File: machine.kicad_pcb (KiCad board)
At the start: 2 copper layers, 69.8 x 69.8 mm, 34 parts, among them J1 TMC2209 Y, J10 SD Card, J11 Stop, J12 Serial, J13 STM32DevV1-VCC, J14 STM32DevV1-3.3, J2 TMC2209 B, J3 X Motor, J4 Y Motor, J5 24V, J6 Buttons, J7 X limit, J8 Y limit, J9 Display, U2 K7805W-500R3

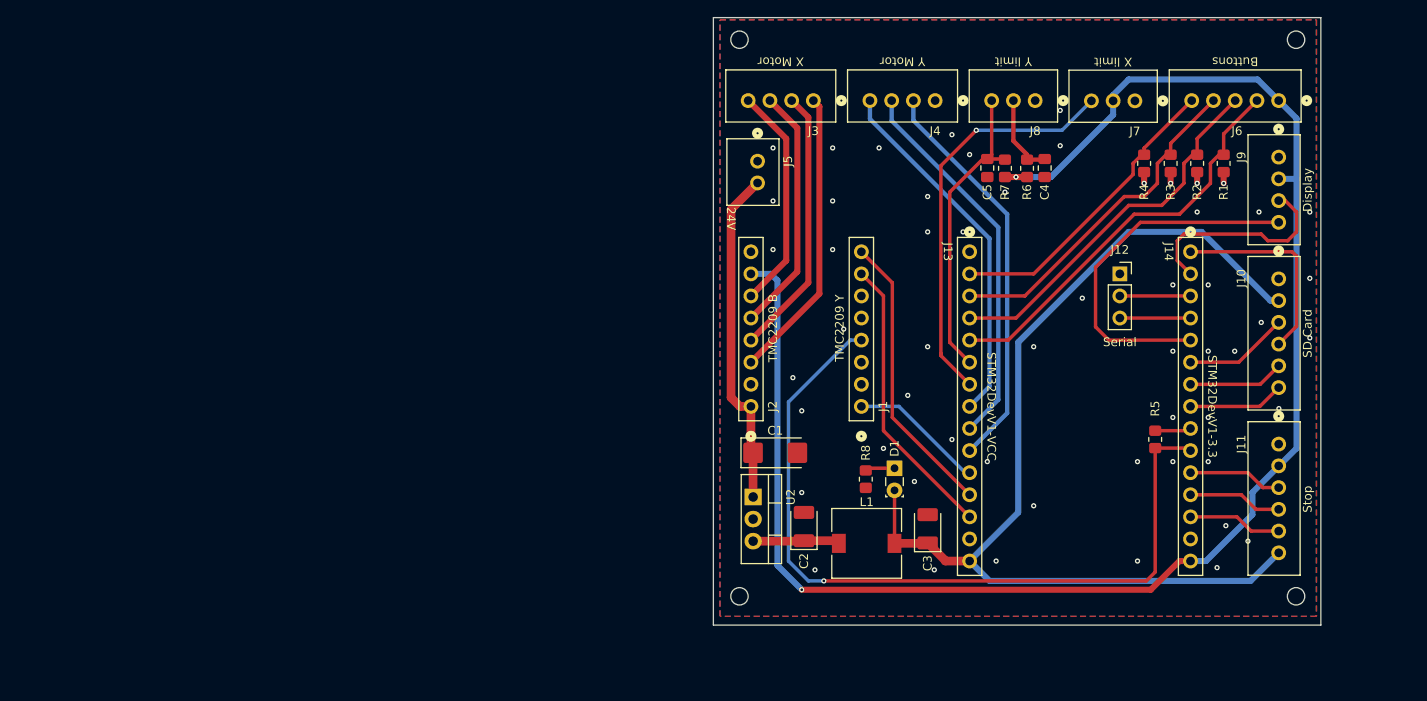
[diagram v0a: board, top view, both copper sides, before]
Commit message: Finalization v2.0
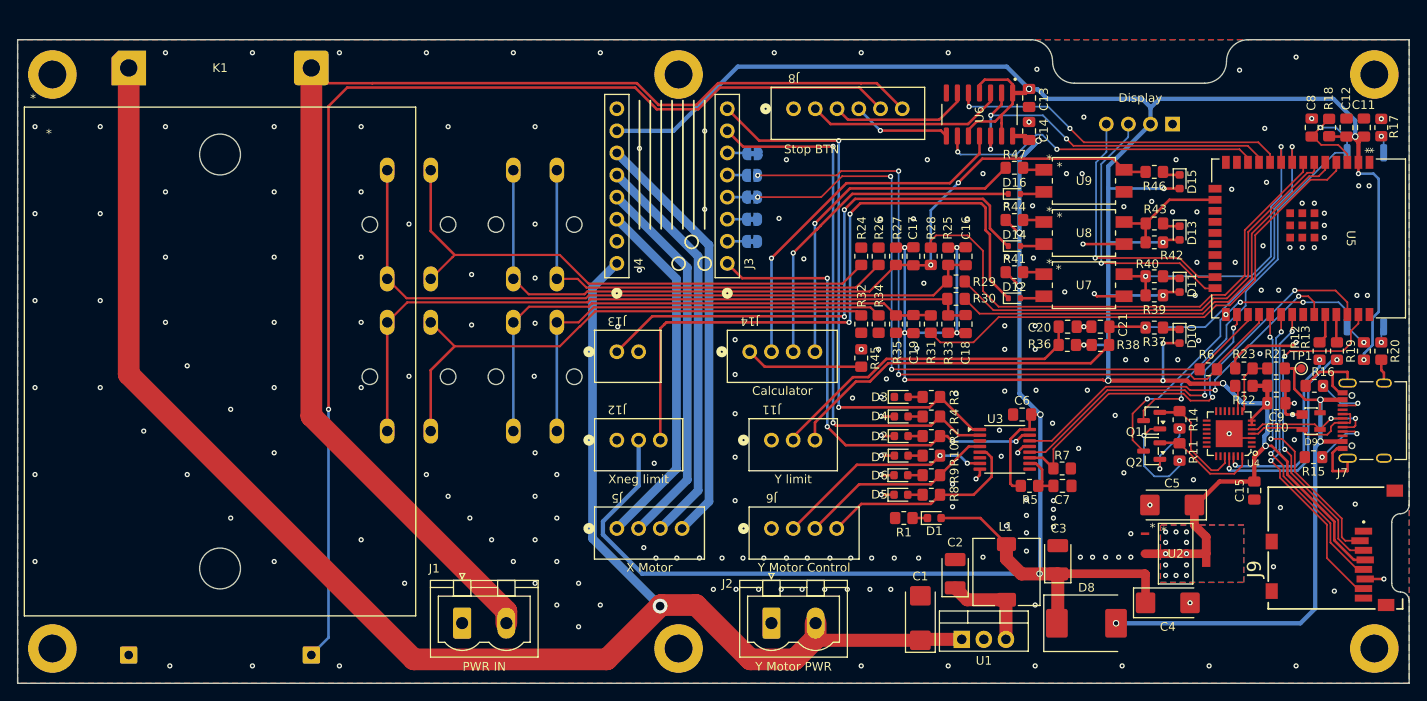
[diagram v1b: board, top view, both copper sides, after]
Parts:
- removed REF** (x4): MountingHole_2mm, MountingHole:MountingHole_2mm
- added C10: 10μF, Capacitor_SMD:C_0805_2012Metric_Pad1.18x1.45mm_HandSolder, F.Cu at (201.7, 86.3)
- added C11: 100nF, Capacitor_SMD:C_0805_2012Metric_Pad1.18x1.45mm_HandSolder, F.Cu at (211.8, 54.6)
- added C12: 22μF, Capacitor_SMD:C_0805_2012Metric_Pad1.18x1.45mm_HandSolder, F.Cu at (209.8, 54.6)
- added C13: 100nF, Capacitor_SMD:C_0805_2012Metric_Pad1.18x1.45mm_HandSolder, F.Cu at (173.3, 51.2)
- added C14: 100nF, Capacitor_SMD:C_0805_2012Metric_Pad1.18x1.45mm_HandSolder, F.Cu at (173.3, 55.0)
- added C15: 100nF, Capacitor_SMD:C_0805_2012Metric_Pad1.18x1.45mm_HandSolder, F.Cu at (199.2, 96.3)
- added C16: 100nF, Capacitor_SMD:C_0805_2012Metric_Pad1.18x1.45mm_HandSolder, F.Cu at (166.0, 69.4)
- added C17: 100nF, Capacitor_SMD:C_0805_2012Metric_Pad1.18x1.45mm_HandSolder, F.Cu at (160.0, 69.4)
- added C18: 100nF, Capacitor_SMD:C_0805_2012Metric_Pad1.18x1.45mm_HandSolder, F.Cu at (166.0, 77.2)
- added C19: 100nF, Capacitor_SMD:C_0805_2012Metric_Pad1.18x1.45mm_HandSolder, F.Cu at (160.0, 77.2)
- added C20: 4.7nF, Capacitor_SMD:C_0805_2012Metric_Pad1.18x1.45mm_HandSolder, F.Cu at (177.7, 77.5)
- added C21: 4.7nF, Capacitor_SMD:C_0805_2012Metric_Pad1.18x1.45mm_HandSolder, F.Cu at (181.5, 77.5)
- added C6: 100nF, Capacitor_SMD:C_0805_2012Metric_Pad1.18x1.45mm_HandSolder, F.Cu at (172.5, 87.6)
- added C7: 100nF, Capacitor_SMD:C_0805_2012Metric_Pad1.18x1.45mm_HandSolder, F.Cu at (177.1, 95.8)
- added C8: 100nF, Capacitor_SMD:C_0805_2012Metric_Pad1.18x1.45mm_HandSolder, F.Cu at (205.8, 54.6)
- added C9: 100nF, Capacitor_SMD:C_0805_2012Metric_Pad1.18x1.45mm_HandSolder, F.Cu at (201.7, 84.3)
- added D10: LED, LED_SMD:LED_0603_1608Metric, F.Cu at (190.6, 78.6)
- added D11: LED, LED_SMD:LED_0603_1608Metric, F.Cu at (190.6, 72.7)
- added D12: RB521S30, Diode_SMD:D_SOD-523, F.Cu at (171.6, 74.2)
- added D13: LED, LED_SMD:LED_0603_1608Metric, F.Cu at (190.6, 66.7)
- added D14: RB521S30, Diode_SMD:D_SOD-523, F.Cu at (171.6, 68.2)
- added D15: LED, LED_SMD:LED_0603_1608Metric, F.Cu at (190.6, 60.8)
- added D16: RB521S30, Diode_SMD:D_SOD-523, F.Cu at (171.6, 62.2)
- added D2: LED, LED_SMD:LED_0603_1608Metric, F.Cu at (158.6, 90.1)
- added D3: LED, LED_SMD:LED_0603_1608Metric, F.Cu at (158.6, 85.6)
- added D4: LED, LED_SMD:LED_0603_1608Metric, F.Cu at (158.6, 87.8)
- added D5: LED, LED_SMD:LED_0603_1608Metric, F.Cu at (158.6, 96.8)
- added D6: LED, LED_SMD:LED_0603_1608Metric, F.Cu at (158.6, 94.6)
- added D7: LED, LED_SMD:LED_0603_1608Metric, F.Cu at (158.6, 92.3)
- added D8: B340A-13-F, Diode_SMD:D_SMC, F.Cu at (179.9, 111.6)
- added D9: SP0503BAHTG, SP0503BAHTG:SOT143, F.Cu at (205.7, 88.4)
- added H1: ~, MountingHole:MountingHole_3.2mm_M3_DIN965_Pad, F.Cu at (61.0, 48.5)
- added H2: ~, MountingHole:MountingHole_3.2mm_M3_DIN965_Pad, F.Cu at (133.0, 48.5)
- added H3: ~, MountingHole:MountingHole_3.2mm_M3_DIN965_Pad, F.Cu at (213.0, 48.5)
- added H4: ~, MountingHole:MountingHole_3.2mm_M3_DIN965_Pad, F.Cu at (213.0, 114.5)
- added H5: ~, MountingHole:MountingHole_3.2mm_M3_DIN965_Pad, F.Cu at (133.0, 114.5)
- added H6: ~, MountingHole:MountingHole_3.2mm_M3_DIN965_Pad, F.Cu at (61.0, 114.5)
- added JP1: PDN, Jumper:SolderJumper-2_P1.3mm_Bridged_RoundedPad1.0x1.5mm, B.Cu at (141.4, 62.6)
- added JP2: PDN, Jumper:SolderJumper-2_P1.3mm_Open_RoundedPad1.0x1.5mm, B.Cu at (141.4, 60.1)
- added JP3: CK, Jumper:SolderJumper-2_P1.3mm_Bridged_RoundedPad1.0x1.5mm, B.Cu at (141.5, 57.6)
- added JP4: MS1, Jumper:SolderJumper-2_P1.3mm_Bridged_RoundedPad1.0x1.5mm, B.Cu at (141.4, 67.7)
- added JP5: MS2, Jumper:SolderJumper-2_P1.3mm_Bridged_RoundedPad1.0x1.5mm, B.Cu at (141.4, 65.2)
- added K1: ZGT-40DD, SSR-DCDC:SSR_DCDC, F.Cu at (57.8, 52.2)
- added Q1: SS8050, Package_TO_SOT_SMD:SOT-23, F.Cu at (187.4, 88.3)
- added Q2: SS8050, Package_TO_SOT_SMD:SOT-23, F.Cu at (187.4, 91.8)
- added R10: 10k, Resistor_SMD:R_0805_2012Metric_Pad1.20x1.40mm_HandSolder, F.Cu at (162.1, 92.3)
- added R11: 10k, Resistor_SMD:R_0805_2012Metric_Pad1.20x1.40mm_HandSolder, F.Cu at (190.6, 91.9)
- added R12: 0, Resistor_SMD:R_0805_2012Metric_Pad1.20x1.40mm_HandSolder, F.Cu at (206.7, 80.3)
- added R13: 0, Resistor_SMD:R_0805_2012Metric_Pad1.20x1.40mm_HandSolder, F.Cu at (208.7, 80.3)
- added R14: 10k, Resistor_SMD:R_0805_2012Metric_Pad1.20x1.40mm_HandSolder, F.Cu at (190.6, 88.2)
- added R15: 5.1k, Resistor_SMD:R_0805_2012Metric_Pad1.20x1.40mm_HandSolder, F.Cu at (206.0, 92.5)
- added R16: 5.1k, Resistor_SMD:R_0805_2012Metric_Pad1.20x1.40mm_HandSolder, F.Cu at (206.1, 84.3)
- added R17: 1k, Resistor_SMD:R_0805_2012Metric_Pad1.20x1.40mm_HandSolder, F.Cu at (213.8, 54.6)
- added R18: 10k, Resistor_SMD:R_0805_2012Metric_Pad1.20x1.40mm_HandSolder, F.Cu at (207.8, 54.6)
- added R19: 10k, Resistor_SMD:R_0805_2012Metric_Pad1.20x1.40mm_HandSolder, F.Cu at (211.8, 80.3)
- added R20: 1k, Resistor_SMD:R_0805_2012Metric_Pad1.20x1.40mm_HandSolder, F.Cu at (213.8, 80.3)
- added R21: 22.1k, Resistor_SMD:R_0805_2012Metric_Pad1.20x1.40mm_HandSolder, F.Cu at (201.7, 82.3)
- added R22: 2k, Resistor_SMD:R_0805_2012Metric_Pad1.20x1.40mm_HandSolder, F.Cu at (198.0, 84.3)
- added R23: 47.5k, Resistor_SMD:R_0805_2012Metric_Pad1.20x1.40mm_HandSolder, F.Cu at (198.0, 82.3)
- added R24: 10, Resistor_SMD:R_0805_2012Metric_Pad1.20x1.40mm_HandSolder, F.Cu at (154.0, 69.4)
- added R25: 1k, Resistor_SMD:R_0805_2012Metric_Pad1.20x1.40mm_HandSolder, F.Cu at (164.0, 69.4)
- added R26: 10, Resistor_SMD:R_0805_2012Metric_Pad1.20x1.40mm_HandSolder, F.Cu at (156.0, 69.4)
- added R27: 1k, Resistor_SMD:R_0805_2012Metric_Pad1.20x1.40mm_HandSolder, F.Cu at (158.0, 69.4)
- added R28: 33, Resistor_SMD:R_0805_2012Metric_Pad1.20x1.40mm_HandSolder, F.Cu at (162.0, 69.4)
- added R29: 33, Resistor_SMD:R_0805_2012Metric_Pad1.20x1.40mm_HandSolder, F.Cu at (164.9, 72.3)
- added R30: 33, Resistor_SMD:R_0805_2012Metric_Pad1.20x1.40mm_HandSolder, F.Cu at (164.9, 74.3)
- added R31: 33, Resistor_SMD:R_0805_2012Metric_Pad1.20x1.40mm_HandSolder, F.Cu at (162.0, 77.2)
- added R32: 10, Resistor_SMD:R_0805_2012Metric_Pad1.20x1.40mm_HandSolder, F.Cu at (154.0, 77.2)
- added R33: 1k, Resistor_SMD:R_0805_2012Metric_Pad1.20x1.40mm_HandSolder, F.Cu at (164.0, 77.2)
- added R34: 10, Resistor_SMD:R_0805_2012Metric_Pad1.20x1.40mm_HandSolder, F.Cu at (156.0, 77.2)
- added R35: 1k, Resistor_SMD:R_0805_2012Metric_Pad1.20x1.40mm_HandSolder, F.Cu at (158.0, 77.2)
- added R36: 200, Resistor_SMD:R_0805_2012Metric_Pad1.20x1.40mm_HandSolder, F.Cu at (177.7, 79.6)
- added R37: 6k8, Resistor_SMD:R_0805_2012Metric_Pad1.20x1.40mm_HandSolder, F.Cu at (187.7, 77.6)
- added R38: 1k2, Resistor_SMD:R_0805_2012Metric_Pad1.20x1.40mm_HandSolder, F.Cu at (181.5, 79.6)
- added R39: 10k, Resistor_SMD:R_0805_2012Metric_Pad1.20x1.40mm_HandSolder, F.Cu at (187.7, 73.9)
- added R40: 6k8, Resistor_SMD:R_0805_2012Metric_Pad1.20x1.40mm_HandSolder, F.Cu at (187.7, 71.7)
- added R41: 680, Resistor_SMD:R_0805_2012Metric_Pad1.20x1.40mm_HandSolder, F.Cu at (171.6, 71.2)
- added R42: 10k, Resistor_SMD:R_0805_2012Metric_Pad1.20x1.40mm_HandSolder, F.Cu at (187.7, 67.8)
- added R43: 6k8, Resistor_SMD:R_0805_2012Metric_Pad1.20x1.40mm_HandSolder, F.Cu at (187.7, 65.6)
- added R44: 680, Resistor_SMD:R_0805_2012Metric_Pad1.20x1.40mm_HandSolder, F.Cu at (171.6, 65.2)
- added R45: 680, Resistor_SMD:R_0805_2012Metric_Pad1.20x1.40mm_HandSolder, F.Cu at (154.0, 81.1)
- added R46: 6k8, Resistor_SMD:R_0805_2012Metric_Pad1.20x1.40mm_HandSolder, F.Cu at (187.7, 59.7)
- added R47: 0, Resistor_SMD:R_0805_2012Metric_Pad1.20x1.40mm_HandSolder, F.Cu at (171.6, 59.2)
- added R9: 10k, Resistor_SMD:R_0805_2012Metric_Pad1.20x1.40mm_HandSolder, F.Cu at (162.1, 94.6)
- added SW1: Reset, Button_Switch_SMD:SW_Push_SPST_NO_Alps_SKRK, B.Cu at (212.0, 57.5)
- added SW2: Boot, Button_Switch_SMD:SW_Push_SPST_NO_Alps_SKRK, B.Cu at (212.0, 77.5)
- added SW3: Run, Button_Switch_THT:SW_SPST_Omron_B3F-40xx, B.Cu at (99.5, 59.5)
- added SW4: Hold, Button_Switch_THT:SW_SPST_Omron_B3F-40xx, B.Cu at (114.0, 59.5)
- added SW5: M2, Button_Switch_THT:SW_SPST_Omron_B3F-40xx, B.Cu at (99.5, 77.0)
- added SW6: M1, Button_Switch_THT:SW_SPST_Omron_B3F-40xx, B.Cu at (114.0, 77.0)
- added TP1: ~, TestPoint:TestPoint_Pad_D1.0mm, F.Cu at (204.6, 82.3)
- added U1: K7805W-500R3, Package_TO_SOT_THT:TO-220-3_Vertical, F.Cu at (165.6, 113.5)
- added U3: 74AHCT595, Package_SO:TSSOP-16_4.4x5mm_P0.65mm, F.Cu at (170.5, 91.6)
- added U4: CP2102-GMR, CP2102_GMR:QFN28G_0.5-5X5MM, F.Cu at (196.3, 89.8)
- added U5: ESP32-WROOM-32E 4MB, ESP32-WROOM-32E-N4:ESP32-WROOM-32E_EXP, F.Cu at (207.2, 67.4)
- added U6: SN74LV125ADR, SN74LV125ADR:SOIC127P600X175-14N, F.Cu at (167.6, 53.1)
- added U7: TLP521-1, TLP521-1XSM:TLP521SM_ISO, F.Cu at (179.6, 72.7)
- added U8: TLP521-1, TLP521-1XSM:TLP521SM_ISO, F.Cu at (179.6, 66.7)
- added U9: TLP521-1, TLP521-1XSM:TLP521SM_ISO, F.Cu at (179.6, 60.7)
- C1: footprint Capacitor_Tantalum_SMD:CP_EIA-6032-28_Kemet-C_Pad2.25x2.35mm_HandSolder -> Capacitor_Tantalum_SMD:CP_EIA-6032-28_Kemet-C_HandSolder
- C2, C3: footprint Capacitor_Tantalum_SMD:CP_EIA-3528-21_Kemet-B_Pad1.50x2.35mm_HandSolder -> Capacitor_Tantalum_SMD:CP_EIA-3528-21_Kemet-B_HandSolder
- C4, C5: value 4.7nF -> 10μF; footprint Capacitor_SMD:C_0805_2012Metric_Pad1.18x1.45mm_HandSolder -> Capacitor_Tantalum_SMD:CP_EIA-6032-28_Kemet-C_HandSolder
- D1: footprint LED_THT:LED_Rectangular_W3.9mm_H1.9mm -> LED_SMD:LED_0603_1608Metric
- J1: value TMC2209 Y -> PWR IN; footprint HDR-08POS:CONN8_LFBN-RC_SUL -> Connector_Phoenix_MSTB:PhoenixContact_MSTBVA_2,5_2-G-5,08_1x02_P5.08mm_Vertical
- J10: value SD Card -> Display; footprint JST-XH-6A:CONN_B6B-XH-A_JST -> Connector_PinSocket_2.54mm:PinSocket_1x04_P2.54mm_Vertical; moved to B.Cu
- J11: value Stop -> Y limit; footprint JST-XH-6A:CONN_B6B-XH-A_JST -> JST-XH-3A:CONN_B3B-XH-A_JST
- J12: value Serial -> Xneg limit; footprint Connector_PinSocket_2.54mm:PinSocket_1x03_P2.54mm_Vertical -> JST-XH-3A:CONN_B3B-XH-A_JST
- J13: value STM32DevV1-VCC -> Xpos limit; footprint HDR-15POS:CONN15_PPPC151LFBN-RC_SUL -> JST-XH-2A:CONN_B2B-XH-A_JST
- J14: value STM32DevV1-3.3 -> Calculator; footprint HDR-15POS:CONN15_PPPC151LFBN-RC_SUL -> JST-XH-4A:CONN_B4B-XH-A_JST
- J2: value TMC2209 B -> Y Motor PWR; footprint HDR-08POS:CONN8_LFBN-RC_SUL -> Connector_Phoenix_MSTB:PhoenixContact_MSTBVA_2,5_2-G-5,08_1x02_P5.08mm_Vertical
- J3: value X Motor -> TMC2209 Y; footprint JST-XH-4A:CONN_B4B-XH-A_JST -> HDR-08POS:CONN8_LFBN-RC_SUL
- J4: value Y Motor -> TMC2209 B; footprint JST-XH-4A:CONN_B4B-XH-A_JST -> HDR-08POS:CONN8_LFBN-RC_SUL
- J5: value 24V -> X Motor; footprint JST-XH-2A:CONN_B2B-XH-A_JST -> JST-XH-4A:CONN_B4B-XH-A_JST
- J6: value Buttons -> Y Motor Control; footprint JST-XH-5A:CONN_B5B-XH-A_JST -> JST-XH-4A:CONN_B4B-XH-A_JST
- J7: value X limit -> TYPE-C 15PIN; footprint JST-XH-3A:CONN_B3B-XH-A_JST -> 10155435_00011LF:AMPHENOL_10155435-00011LF
- J8: value Y limit -> Stop BTN; footprint JST-XH-3A:CONN_B3B-XH-A_JST -> JST-XH-6A:CONN_B6B-XH-A_JST
- J9: value Display -> Int SD; footprint JST-XH-4A:CONN_B4B-XH-A_JST -> MEM2061_01_188_00_A:GCT_MEM2061-01-188-00-A_REVA
- R1, R2, R3, R4: value 47k -> 10k
- R5: value 1k -> 10k
- R6: value 200 -> 1k
- R7: value 1.2k -> 10k
- R8: value 3.3k -> 10k
- U2: value K7805W-500R3 -> NCP1117IST33T3G; footprint Package_TO_SOT_THT:TO-220-3_Vertical -> NCP1117IST33T3G:SOT-223_NCP1117IST33T3G_OSI
- moved J6 76.3 mm to (143.7, 100.7), turned to 180 degrees
- moved J12 60.9 mm to (125.9, 90.5), turned to 180 degrees
- moved J11 58.3 mm to (143.7, 90.5), turned to 180 degrees
- moved R1 54.9 mm to (158.9, 99.5), turned to 180 degrees
- moved J1 52.2 mm to (108.1, 111.6), turned to 0 degrees
- moved J14 52.0 mm to (141.2, 80.4), turned to 180 degrees
- moved C4 52.0 mm to (189.2, 109.2), turned to 0 degrees
- moved U2 49.0 mm to (190.2, 103.6), turned to 0 degrees
- moved J7 46.6 mm to (214.1, 88.3), turned to 90 degrees
- moved J9 45.4 mm to (208.5, 103.0)
- moved J5 45.2 mm to (125.9, 100.7), turned to 180 degrees
- moved C5 44.2 mm to (189.8, 98.0), turned to 180 degrees
- moved R2 43.8 mm to (162.1, 90.1), turned to 180 degrees
- moved J13 42.2 mm to (125.9, 80.4), turned to 180 degrees
- moved J4 41.1 mm to (125.9, 70.2), turned to 90 degrees
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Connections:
- C2 pad 1: Net-(U2-VO) -> Net-(U1-VO)
- C4 pad 1: GND -> +5V
- C4 pad 2: /VH -> GND
- C5 pad 1: GND -> +3V3
- C5 pad 2: /GPIO32 -> GND
- J1 pad 1: /ENX -> GND
- J1 pad 2: GND -> VCC
- J10 pad 2: +5V -> +3V3
- J10 pad 3: /GPIO19 -> D_SCK
- J10 pad 4: /GPIO23 -> D_SDA
- J11 pad 2: 3.3V -> /IO/VH
- J11 pad 3: /GPIO4 -> Y_ALL_LIM
- J12 pad 2: /GPIO1 -> +5V
- J12 pad 3: /GPIO3 -> /IO/QXneg
- J13 pad 1: unconnected-(J13-Pad1) -> /IO/QXpos
- J13 pad 2: /GPIO36 -> GND
- J14 pad 1: /GPIO23 -> Net-(J14-Pad1)
- J14 pad 2: /GPIO22 -> RUN
- J14 pad 3: /GPIO1 -> CGND
- J14 pad 4: /GPIO3 -> Net-(J14-Pad4)
- J2 pad 1: 24V -> GND
- J2 pad 2: GND -> 24V
- J3 pad 1: /A2 -> /Power/X_ENABLE
- J3 pad 2: /A1 -> /Power/MS1
- J3 pad 3: /B1 -> /Power/MS2
- J3 pad 4: /B2 -> /Power/PDN (TX)
- J4 pad 1: GND -> 24V
- J4 pad 2: /ENY -> GND
- J4 pad 3: /DIRY -> /Power/A2
- J4 pad 4: /GPIO25 -> /Power/A1
- J5 pad 1: GND -> /Power/A2
- J5 pad 2: 24V -> /Power/A1
- J6 pad 1: 3.3V -> GND
- J6 pad 2: /GPIO35 -> /Power/Y_ENABLE
- J6 pad 3: /GPIO34 -> /Power/Y_DIR
- J6 pad 4: /GPIO39 -> /Power/Y_STEP
- J8 pad 2: /VH -> /IO/L_RUN
- J8 pad 3: /GPIO32 -> /IO/L_HOLD
- J9 pad 1: GND -> unconnected-(J9-DAT2-Pad1)
- J9 pad 2: 3.3V -> SD_CS
- J9 pad 3: /GPIO22 -> SD_MOSI
- J9 pad 4: /GPIO21 -> +3V3
- L1 pad 1: Net-(U2-VO) -> Net-(U1-VO)
- R1 pad 1: GND -> Net-(D1-K)
- R1 pad 2: /GPIO35 -> GND
- R2 pad 1: GND -> /Power/X_ENABLE
- R2 pad 2: /GPIO34 -> Net-(D2-A)
- R3 pad 1: GND -> /Power/X_DIR
- R3 pad 2: /GPIO39 -> Net-(D3-A)
- R4 pad 1: GND -> /Power/X_STEP
- R4 pad 2: /GPIO36 -> Net-(D4-A)
- R5 pad 1: /GPIO17 -> Net-(U3-~{SRCLR})
- R5 pad 2: /GPIO16 -> +5V
- R6 pad 1: /VH -> X_RXD
- R6 pad 2: 3.3V -> X_TXD
- R7 pad 1: /GPIO32 -> GND
- R7 pad 2: 3.3V -> I2S_BCK
- R8 pad 1: Net-(D1-K) -> Net-(D5-A)
- R8 pad 2: GND -> /Power/Y_STEP
- U2 pad 1: 24V -> GND
- U2 pad 2: GND -> +3V3
- U2 pad 3: Net-(U2-VO) -> +5V
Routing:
- net +3V3: track 0.00 -> 353.4 mm, vias 0 -> 31
- net 3.3V: track 187.8 -> 0.00 mm, vias 2 -> 0
- net 24V: track 39.2 -> 196.4 mm, vias 0 -> 1
- net VCC: track 0.00 -> 145.1 mm
- net PWR SW: track 0.00 -> 131.4 mm, vias 0 -> 1
- net HOLD: track 0.00 -> 96.7 mm, vias 0 -> 2
- net /GPIO16: track 91.6 -> 0.00 mm, vias 1 -> 0
- net X_TXD: track 0.00 -> 85.4 mm, vias 0 -> 3
- net Net-(C16-Pad1): track 0.00 -> 82.6 mm
- net X_RXD: track 0.00 -> 82.5 mm, vias 0 -> 3
- net Net-(C18-Pad2): track 0.00 -> 82.0 mm
- net Y_ALL_LIM: track 0.00 -> 79.4 mm, vias 0 -> 2
- net /IO/QXneg: track 0.00 -> 75.2 mm, vias 0 -> 2
- net Net-(R24-Pad2): track 0.00 -> 63.8 mm
- net Net-(R32-Pad1): track 0.00 -> 63.4 mm
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- added copper zone on B.Cu, net +3V3
- added copper zone on F.Cu, net +3V3
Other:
- board size 69.8 x 69.8 mm -> 160 x 74 mm
- board text added: "Rapunceḷ Dyzajn HW Version: 2.0"
